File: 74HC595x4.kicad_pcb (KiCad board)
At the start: 2 copper layers, 49 parts, among them P1 CONN_01X06, P2 CONN_02X08, P3 CONN_02X08, P4 CONN_02X08, P5 CONN_02X08, U1 74HC595, U2 74HC595, U3 74HC595, U4 74HC595

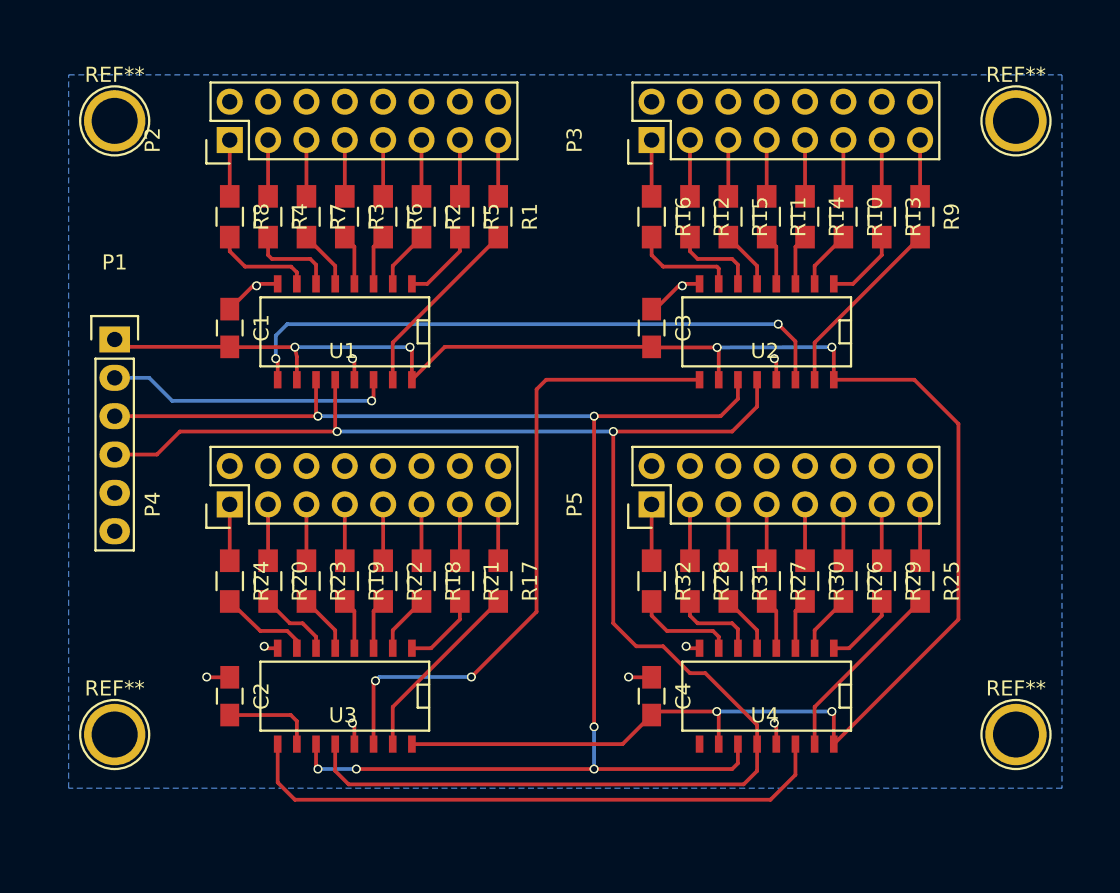
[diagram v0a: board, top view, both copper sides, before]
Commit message: пред готовность. толстые питающие метрические размеры
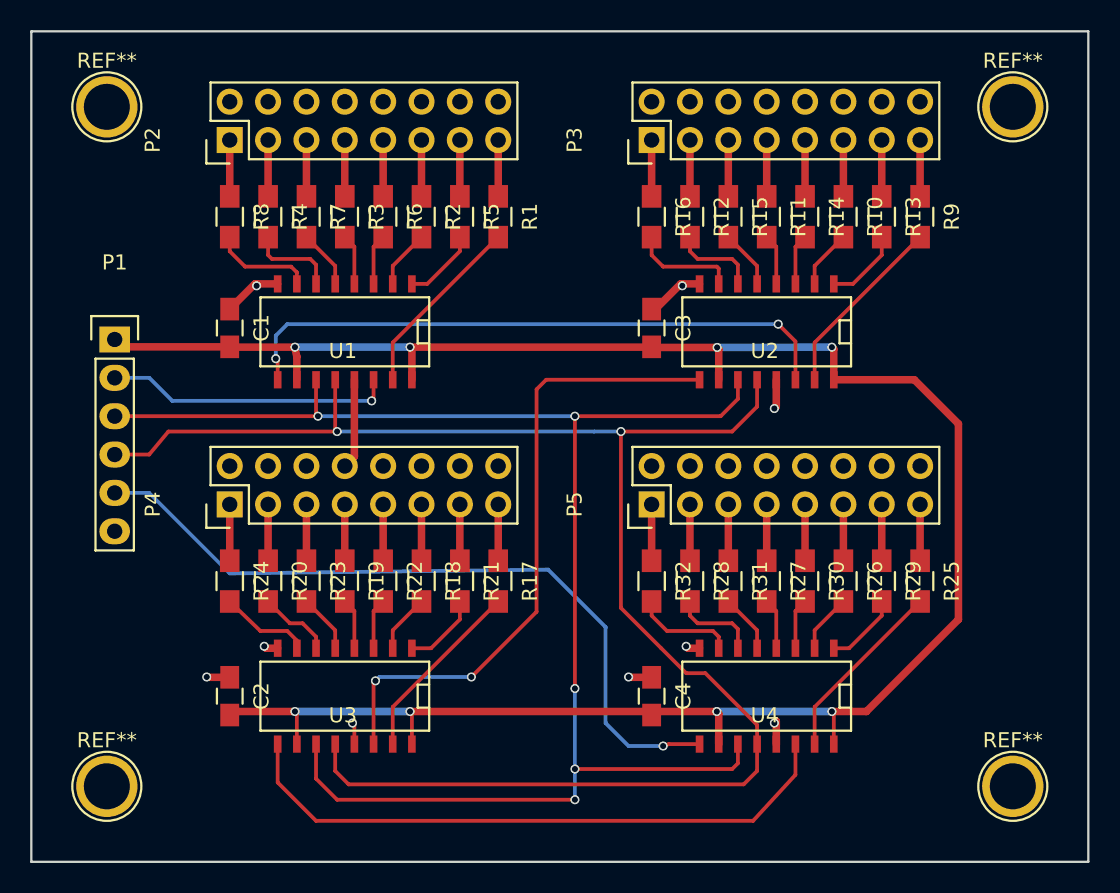
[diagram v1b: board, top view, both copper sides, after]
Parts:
- moved REF** 3.47 mm to (96.0, 119.0)
- moved REF** 3.44 mm to (156.0, 119.0)
- moved REF** 1.07 mm to (96.0, 74.0)
- moved REF** 0.95 mm to (156.0, 74.0)
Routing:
- net /74HC595_4/~Q7: track 0.00 -> 49.5 mm, vias 0 -> 1
- net VCC: track 131.4 -> 139.7 mm, vias 6 -> 8
- net GND: track 19.9 -> 24.4 mm, vias 10 -> 9
- net /74HC595_1/SH_CP: track 99.8 -> 103.1 mm, vias 6 -> 5
- net /74HC595_4/DS: track 40.0 -> 41.3 mm
- net /74HC595_1/ST_CP: track 107.9 -> 106.9 mm
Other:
- board outline added: 70 x 55 mm
- net class power added: clearance 0.2, trace_width 0.5, via_dia 0.6, via_drill 0.4
